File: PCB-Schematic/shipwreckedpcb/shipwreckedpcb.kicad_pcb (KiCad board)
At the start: 4 copper layers, 61.8 x 79.6 mm, 180 parts, among them J1 USB4105, J14 Conn_01x01, J15 Conn_01x01, J16 Conn_01x01, J17 Conn_01x01, J18 Conn_01x01, J19 Conn_01x01, J2 Waveshare 1.54" E-Ink, J20 Conn_01x01, J21 Conn_01x01, J22 Conn_01x01, J23 Conn_01x01, J24 Conn_01x01, J25 Conn_01x01, J26 Conn_01x01, J28 Conn_01x01, J29 Conn_01x01, J3 Conn_01x01, J30 Conn_01x01, J31 Conn_01x01, J32 Conn_01x01, J33 Conn_01x01, J34 Conn_01x01, J35 Conn_01x01, J36 Conn_01x01, J37 Conn_01x01, J38 Conn_01x01, J39 Conn_01x01, J4 Conn_01x01, J5 SWD, J6 Conn_01x01, J7 Conn_01x01, Q1 Si1308EDL, SW1 BOOTSEL, SW10 Resistive, SW11 Clicky - THT, SW12 Clicky - SMD, SW13 Clicky - THT, SW14 Clicky - SMD, SW15 Clicky - THT, SW16 Clicky - SMD, SW17 Clicky - THT, SW18 Clicky - SMD, SW19 PWR Switch, SW2 RESET, SW3 Resistive, SW4 Resistive, SW5 Resistive, SW6 Resistive, SW7 Resistive, SW8 Resistive, SW9 Resistive, U1 RP2040, U2 W25Q128JVS, U3 Si4463, U4 TPS61200DRC, U5 AS179-92LF, U7 PCA9555PW, U8 ST25DV04K-IE6S3, Y1 ABM8-272-T3, Y2 X322530MOB4SI

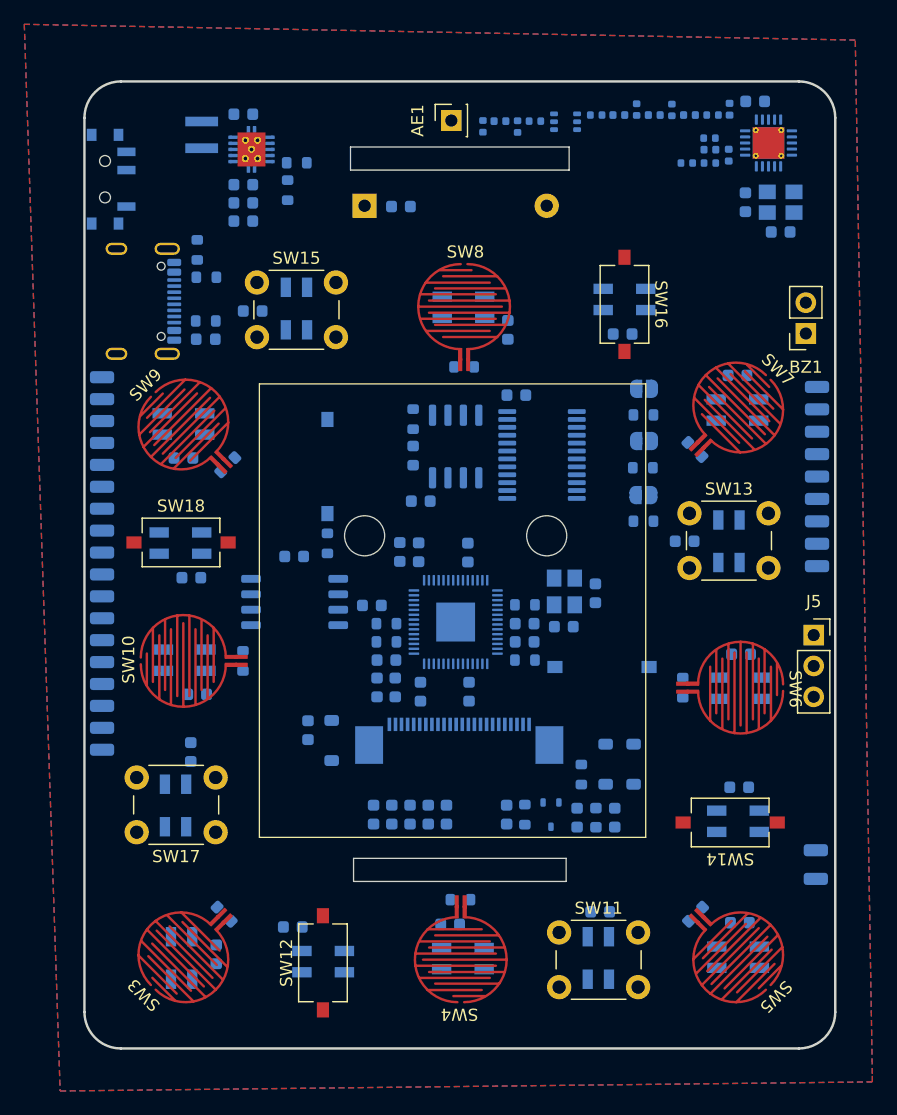
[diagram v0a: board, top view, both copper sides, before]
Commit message: start routing
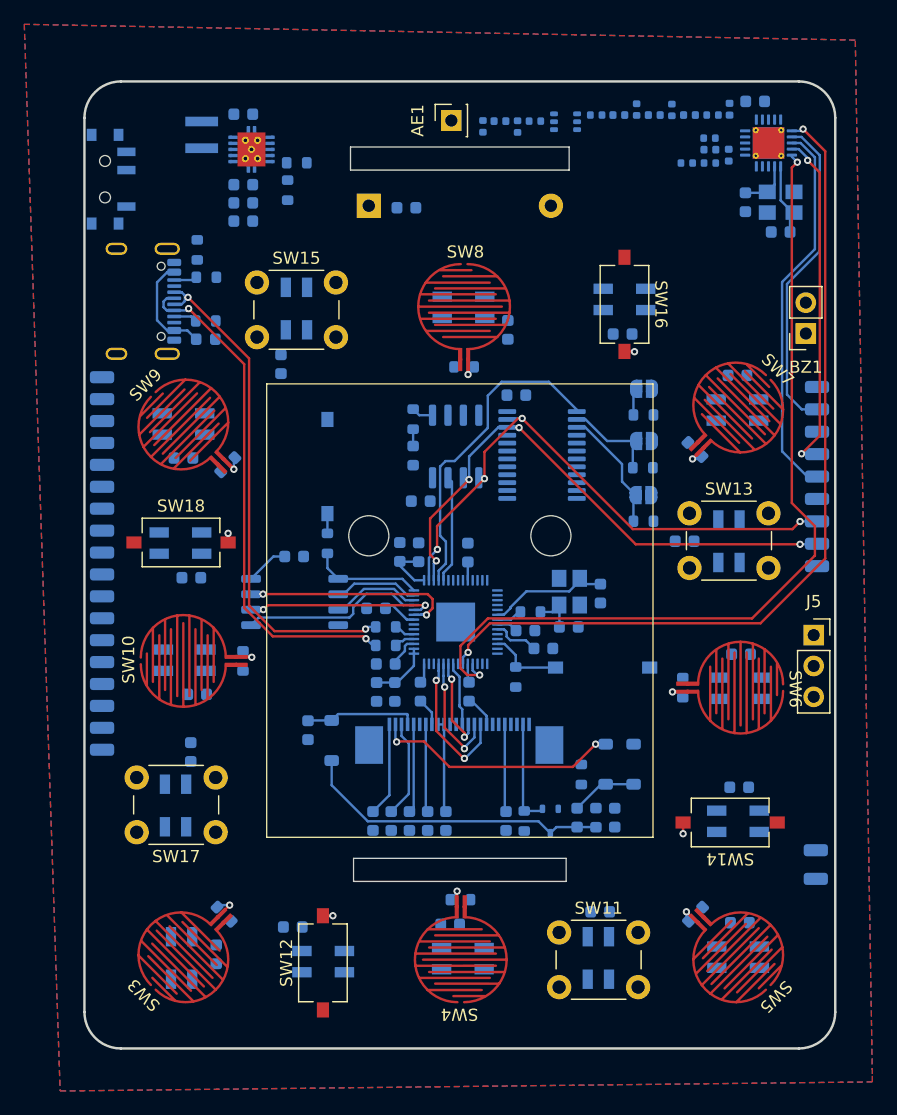
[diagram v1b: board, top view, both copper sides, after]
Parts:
- moved C29 4.95 mm to (132.3, 85.4), turned to -90 degrees
- moved C2 1.64 mm to (153.9, 108.8)
- moved R6 1.59 mm to (151.7, 111.2), turned to 90 degrees
- moved R1 0.74 mm to (152.9, 105.8)
- moved C7 0.57 mm to (152.4, 107.3)
- moved C15 0.53 mm to (150.8, 123.0)
- moved Q1 0.53 mm to (154.5, 123.0)
- moved R9 0.53 mm to (152.3, 123.0)
- moved C16 0.53 mm to (145.9, 123.0)
- moved C17 0.53 mm to (144.4, 123.0)
- moved C18 0.53 mm to (142.9, 123.0)
- moved C19 0.53 mm to (141.4, 123.0)
- moved C20 0.53 mm to (139.9, 123.0)
- moved C51 0.46 mm to (142.7, 72.5)
- moved C1 0.42 mm to (140.2, 105.5)
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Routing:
- net /SI_NSEL: track 0.00 -> 71.3 mm, vias 0 -> 2
- net /SI_NIRQ: track 0.00 -> 71.2 mm, vias 0 -> 2
- net /I2C_SDA: track 0.00 -> 46.8 mm, vias 0 -> 4
- net /I2C_SCL: track 0.00 -> 46.0 mm, vias 0 -> 4
- net /USB_DM: track 0.00 -> 42.3 mm, vias 0 -> 2
- net /USB_DP: track 0.00 -> 41.7 mm, vias 0 -> 2
- net /SPI_MISO: track 0.00 -> 31.4 mm
- net /SPI_MOSI: track 0.00 -> 28.3 mm, vias 0 -> 2
- net /SPI_CLK: track 0.00 -> 26.7 mm
- net /IO_INT: track 0.00 -> 26.6 mm
- net Net-(D4-A): track 0.00 -> 25.6 mm
- net /DISP_PREVGL: track 0.00 -> 20.3 mm, vias 0 -> 2
- net +3V3: track 0.00 -> 19.4 mm
- net /QSPI_SD3: track 0.00 -> 17.9 mm, vias 0 -> 2
- net /QSPI_SCLK: track 0.00 -> 15.6 mm, vias 0 -> 2
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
